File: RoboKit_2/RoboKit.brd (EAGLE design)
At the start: 134 x 82 mm, 28 parts, among them P1 B6B-PH-K, P2 B6B-PH-K, U1 CD74HC4067SM96, X1 JST-XH-03-PIN-LONG-PAD, X2 JST-XH-02-PIN-LONG-PAD, X3 JST-XH-02-PIN-LONG-PAD, X4 JST-XH-02-PIN-LONG-PAD, X5 JST-XH-04-PIN-LONG-PAD, X6 JST-XH-04-PIN-LONG-PAD, X7 JST-XH-10-PIN-LONG-PAD, X8 JST-XH-02-PIN-LONG-PAD, X9 JST-XH-03-PIN-LONG-PAD

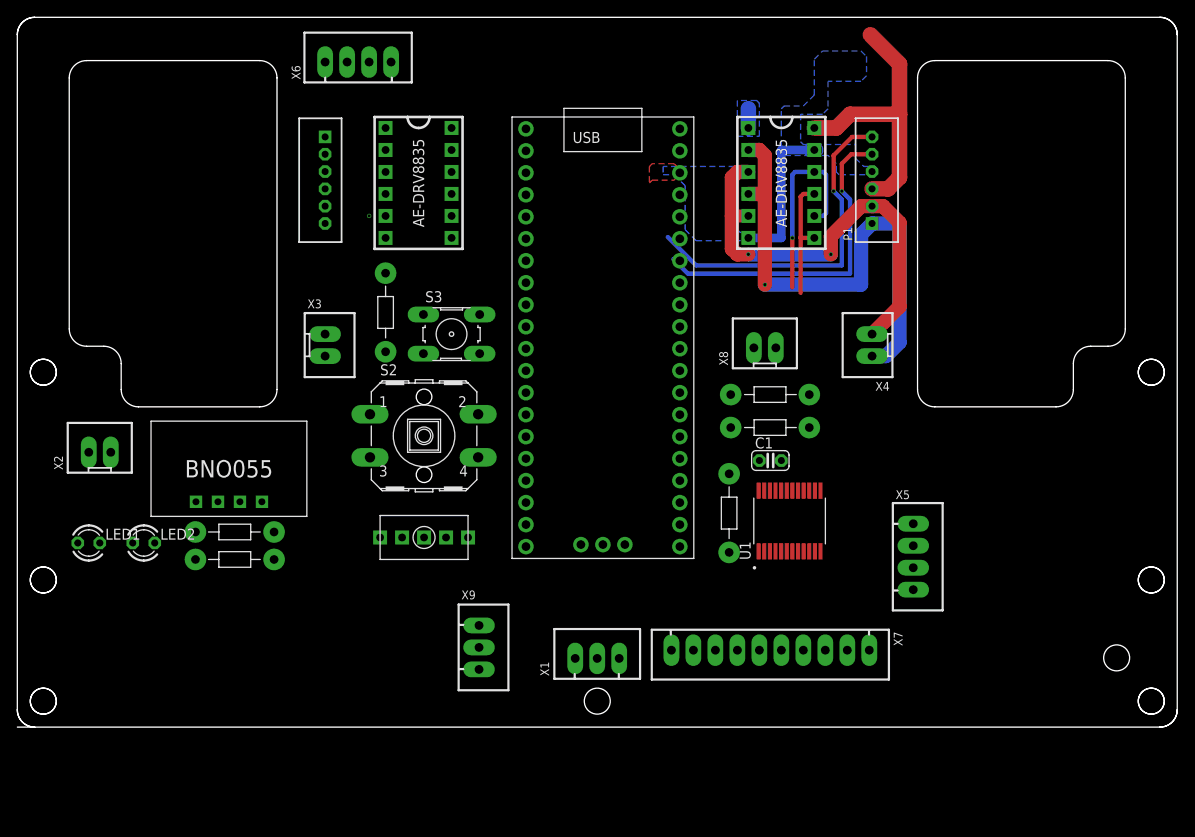
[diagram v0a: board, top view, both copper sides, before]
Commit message: とりあえず完成！
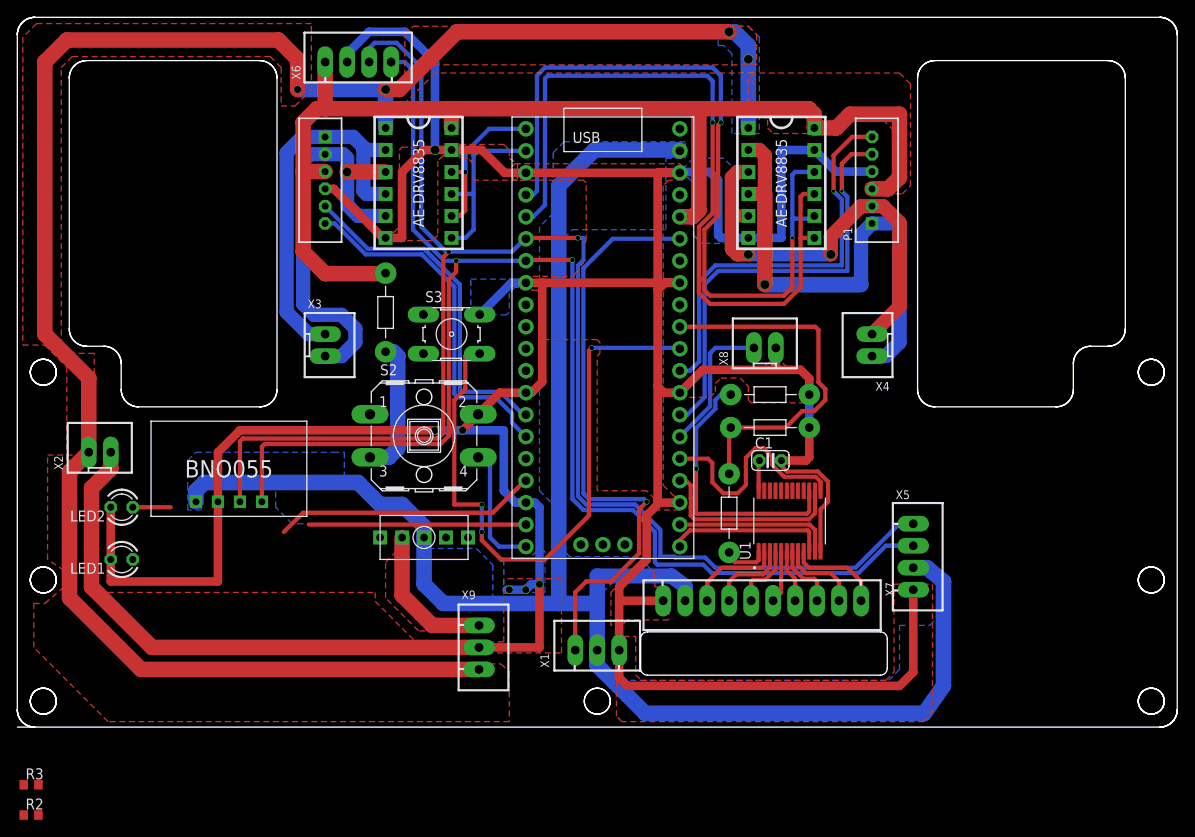
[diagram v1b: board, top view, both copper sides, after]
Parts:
- removed CONNECTOR2, CONNECTOR3: RESISTER, resistor:RESISTER_SOCKET
- added R2, R3: (no value), rcl:R0603
- moved X7 5.79 mm to (86.0, 14.6)
- moved LED2 4.85 mm to (12.1, 25.4), turned to 180 degrees
- moved LED1 4.26 mm to (12.1, 19.4), turned to 180 degrees
- moved X1 0.95 mm to (67.0, 8.89)
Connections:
- new net $10: C1.1, U1.24
- net 0X: now also X7.1; no longer X7.3
- net 0Y: now also X7.5; no longer X7.7
- net 1X: now also X7.2; no longer X7.4
- net 1Y: now also X7.6; no longer X7.8
- net 2X: now also X7.3; no longer X7.5
- net 2Y: now also X7.7; no longer X7.9
- net 3X: now also X7.4; no longer X7.6
- net 3Y: now also X7.8; no longer X7.10
- net GND: now also X7.10; no longer X7.1
- net HALL_A_L: now also U$1.14; no longer U$1.27
- net HALL_A_R: now also U$1.27; no longer U$1.14
- net HALL_B_L: now also U$1.15; no longer U$1.29
- net HALL_B_R: now also U$1.29; no longer U$1.15
- net IO13: now also R3.2; no longer CONNECTOR3.2
- net IO14: now also R2.2; no longer CONNECTOR2.2
- net IO20: now also X8.1
- net IO7: no longer X8.1
- net N$1: now also R2.1; no longer CONNECTOR2.1
- net N$3: now also R3.1; no longer CONNECTOR3.1
- net VSYS: now also X7.9; no longer C1.1, U1.24, X7.2
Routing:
- net GND: track 17.8 -> 506.0 mm, vias 0 -> 6
- net VOUT: track 2.22 -> 220.1 mm, vias 0 -> 4
- net VSYS: track 0.00 -> 204.5 mm
- net SDA: track 0.00 -> 176.6 mm, vias 0 -> 2
- net SCL: track 0.00 -> 164.3 mm, vias 0 -> 2
- net 3V3: track 32.1 -> 133.3 mm
- net IO3: track 14.4 -> 89.1 mm, vias 0 -> 1
- net RUN: track 0.00 -> 71.9 mm, vias 0 -> 3
- net ANALOG: track 0.00 -> 68.5 mm, vias 0 -> 1
- net IO2: track 23.1 -> 91.5 mm, vias 1 -> 2
- net MOTOR_B_L: track 0.00 -> 49.9 mm
- net MOTOR_A_L: track 0.00 -> 44.5 mm
- net Y-COM: track 0.00 -> 42.3 mm
- net HALL_B_L: track 0.00 -> 41.3 mm
- net HALL_A_L: track 0.00 -> 40.4 mm
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- added copper zone on layer 1, net 3V3
- added copper zone on layer 1, net 5.0V
- added copper zone on layer 1, net VOUT
- added copper zone on layer 16, net VSYS
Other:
- outline, holes or cut-outs redrawn
